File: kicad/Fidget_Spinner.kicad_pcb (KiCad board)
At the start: 2 copper layers, 117.7 x 106.2 mm, 29 parts, among them Q1 BC846, U1 BAT_HLD_SMD, U2 BAT_HLD_SMD, U3 BAT_HLD_SMD

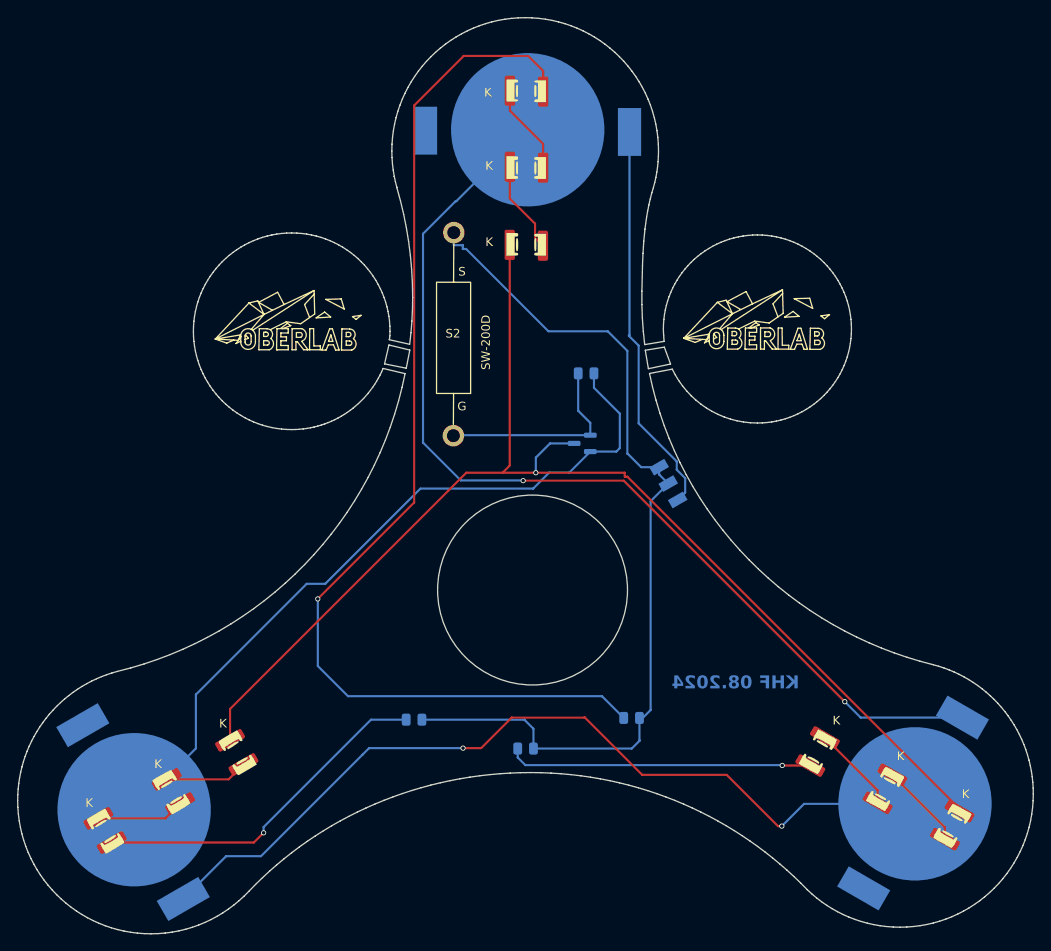
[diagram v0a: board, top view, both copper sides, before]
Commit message: V 19.08.2024
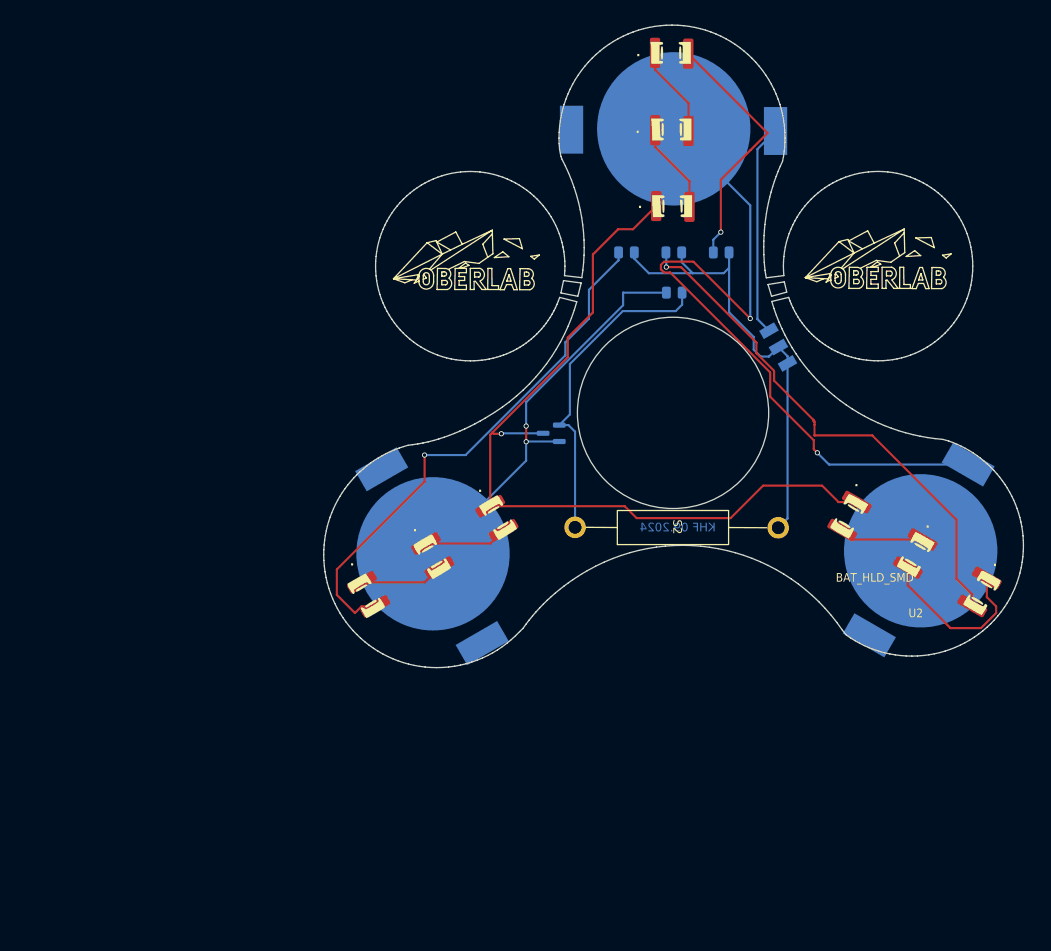
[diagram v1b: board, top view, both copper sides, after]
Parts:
- removed the G*** at (91.4, 73.3)
- removed the G*** at (64.4, 94.3) (x6)
- removed the G*** at (37.0, 73.4)
- removed the G*** at (97.0, 89.2)
- removed the G*** at (42.6, 89.6)
- added G***: LOGO, !Goody:ob-logo_B.SilkS, F.Cu at (63.3, 82.4)
- added G*** (x6): LOGO, LOGO, F.Cu at (83.2, 73.9)
- added G***: LOGO, !Goody:ob-logo_B.SilkS, F.Cu at (111.0, 82.2)
- added G***: LOGO, !Goody:ob-logo_F.SilkS, F.Cu at (105.5, 66.3)
- added G***: LOGO, !Goody:ob-logo_F.SilkS, F.Cu at (57.7, 66.4)
- moved R2 60.0 mm to (81.7, 64.4)
- moved R3 59.5 mm to (76.2, 64.4)
- moved R1 55.0 mm to (87.2, 64.4)
- moved U3 45.6 mm to (53.5, 99.4)
- moved D8 45.4 mm to (56.2, 98.7), turned to 0 degrees
- moved D7 41.0 mm to (48.8, 103.2)
- moved D9 40.6 mm to (63.6, 94.4)
- moved D6 37.8 mm to (106.1, 93.9)
- moved S2 33.6 mm to (81.6, 96.2), turned to -90 degrees
- moved D5 31.6 mm to (113.8, 98.3), turned to 0 degrees
- moved U2 29.3 mm to (109.5, 99.6)
- moved D4 26.4 mm to (121.2, 102.7)
- moved S1 20.3 mm to (93.8, 75.3), turned to 0 degrees
- moved D2 19.8 mm to (82.8, 50.8), turned to 0 degrees
- moved D3 17.6 mm to (82.9, 59.6)
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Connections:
- D2 pad 1: Net-(D1-K) -> Net-(D2-K)
- D2 pad 2: Net-(D2-K) -> Net-(D1-K)
- D5 pad 1: Net-(D4-K) -> Net-(D5-K)
- D5 pad 2: Net-(D5-K) -> Net-(D4-K)
- D8 pad 1: Net-(D7-K) -> Net-(D8-K)
- D8 pad 2: Net-(D8-K) -> Net-(D7-K)
- U3 pad 1: unconnected-(U2-Pad2) -> unconnected-(U3-Pad1)
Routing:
- net unconnected-(U2-Pad2): track 99.8 -> 0.00 mm, vias 2 -> 0
- net Net-(D1-A): track 128.0 -> 29.5 mm
- net Net-(D3-K): track 149.9 -> 95.2 mm
- net Net-(S1-E): track 105.3 -> 53.6 mm
- net Net-(Q1-E): track 87.0 -> 48.3 mm, vias 0 -> 2
- net Net-(U1-Pad2): track 117.1 -> 86.7 mm
- net Net-(D4-A): track 35.3 -> 60.7 mm
- net Net-(D7-A): track 40.4 -> 61.7 mm
- net Net-(S1-A-Pad1): track 45.8 -> 24.6 mm
- net Net-(Q1-B): track 23.6 -> 38.1 mm
- net Net-(D4-K): track 10.1 -> 19.6 mm
- net Net-(D7-K): track 10.2 -> 9.67 mm
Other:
- board size 117.7 x 106.2 mm -> 81.1 x 74.5 mm
- board text added: "."
- board text added: "KHF 09.2024"
- board text removed: "150R"
- board text removed: "1k"
- board text removed: "B"
- board text removed: "BC846B"
- board text removed: "C"
- board text removed: "E"
- board text removed: "G"
- board text removed: "JLCJLCJLCJLC"
- board text removed: "K"
- board text removed: "KHF 08.2024"
- board text removed: "R2"
- board text removed: "S"
- board text removed: "SW-200D"
